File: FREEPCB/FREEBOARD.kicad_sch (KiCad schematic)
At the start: 370 parts, among them J1 OLED_DISPLAY, SW1 SW_Push_45deg, SW10 SW_Push_45deg, SW11 SW_Push_45deg, SW12 SW_Push_45deg, SW13 SW_Push_45deg, SW14 SW_Push_45deg, SW15 SW_Push_45deg, SW16 SW_Push_45deg, SW17 SW_Push_45deg, SW18 SW_Push_45deg, SW19 SW_Push_45deg, SW2 SW_Push_45deg, SW20 SW_Push_45deg, SW21 SW_Push_45deg, SW22 SW_Push_45deg, SW23 SW_Push_45deg, SW24 SW_Push_45deg, SW25 SW_Push_45deg, SW26 SW_Push_45deg, SW27 SW_Push_45deg, SW28 SW_Push_45deg, SW29 SW_Push_45deg, SW3 SW_Push_45deg, SW30 SW_Push_45deg, SW31 SW_Push_45deg, SW32 SW_Push_45deg, SW33 SW_Push_45deg, SW34 SW_Push_45deg, SW35 SW_Push_45deg, SW36 SW_Push_45deg, SW37 SW_Push_45deg, SW38 SW_Push_45deg, SW39 SW_Push_45deg, SW4 SW_Push_45deg, SW40 SW_Push_45deg, SW41 SW_Push_45deg, SW42 SW_Push_45deg, SW43 SW_Push_45deg, SW44 SW_Push_45deg, SW45 SW_Push_45deg, SW46 SW_Push_45deg, SW47 SW_Push_45deg, SW48 SW_Push_45deg, SW49 SW_Push_45deg, SW5 SW_Push_45deg, SW50 SW_Push_45deg, SW51 SW_Push_45deg, SW52 SW_Push_45deg, SW53 SW_Push_45deg, SW54 SW_Push_45deg, SW55 SW_Push_45deg, SW56 SW_Push_45deg, SW57 SW_Push_45deg, SW58 SW_Push_45deg, SW59 SW_Push_45deg, SW6 SW_Push_45deg, SW60 SW_Push_45deg, SW61 SW_Push_45deg, SW62 SW_Push_45deg, SW63 SW_Push_45deg, SW64 SW_Push_45deg, SW65 SW_Push_45deg, SW66 SW_Push_45deg, SW67 SW_Push_45deg, SW68 SW_Push_45deg, SW69 SW_Push_45deg, SW7 SW_Push_45deg, SW70 SW_Push_45deg, SW71 SW_Push_45deg, SW72 SW_Push_45deg, SW73 SW_Push_45deg, SW74 SW_Push_45deg, SW75 SW_Push_45deg, SW76 SW_Push_45deg, SW77 SW_Push_45deg, SW78 SW_Push_45deg, SW79 SW_Push_45deg, SW8 SW_Push_45deg, SW80 SW_Push_45deg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

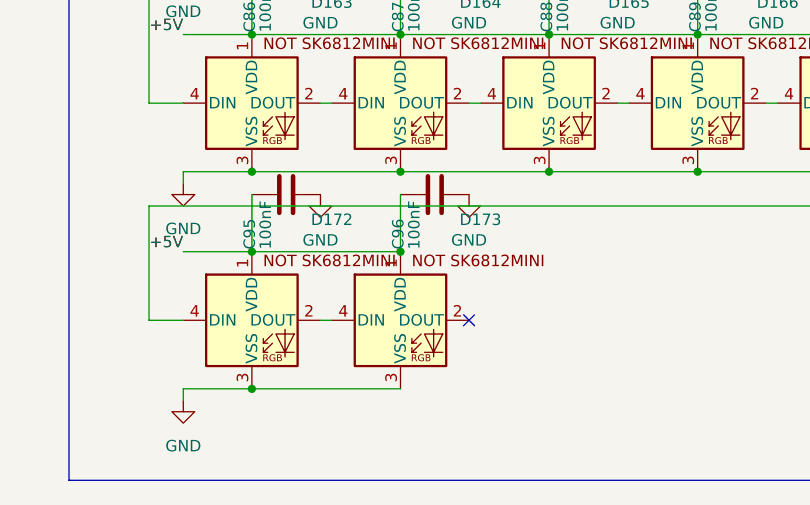
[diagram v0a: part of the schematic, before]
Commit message: PCB Update
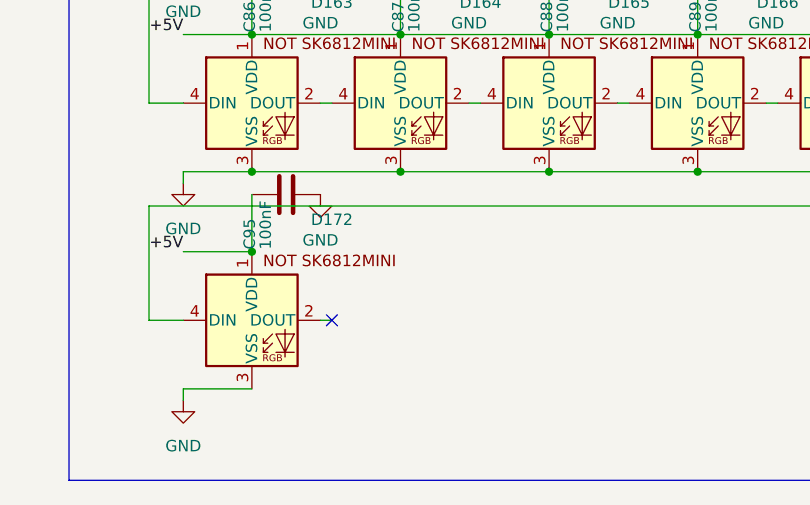
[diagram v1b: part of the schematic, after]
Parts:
- removed C96: 100nF, Capacitor_SMD:C_0603_1608Metric_Pad1.08x0.95mm_HandSolder, symbol Device:C
- removed D173: SK6812MINI-E, footprints:SK6812MINI-E_fixed, symbol SK6812MINI-E:SK6812MINI-E
- J1: footprint KiCad-SSD1306-0.91-OLED-4pin-128x32.pretty-master:SSD1306-0.91-OLED-4pin-128x32 -> Connector_JST:JST_SH_BM04B-SRSS-TB_1x04-1MP_P1.00mm_Vertical
